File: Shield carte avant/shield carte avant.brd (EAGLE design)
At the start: 68.6 x 53.3 mm, 29 parts, among them IC1 MCP2562-E_P, IC2 MCP2515-I_P, J1 22-05-7078-07, J2 22-05-7028-02, J3 22-05-7038-03, J5 22-05-7028-02, M1 ARDUINO_R3_ICSP

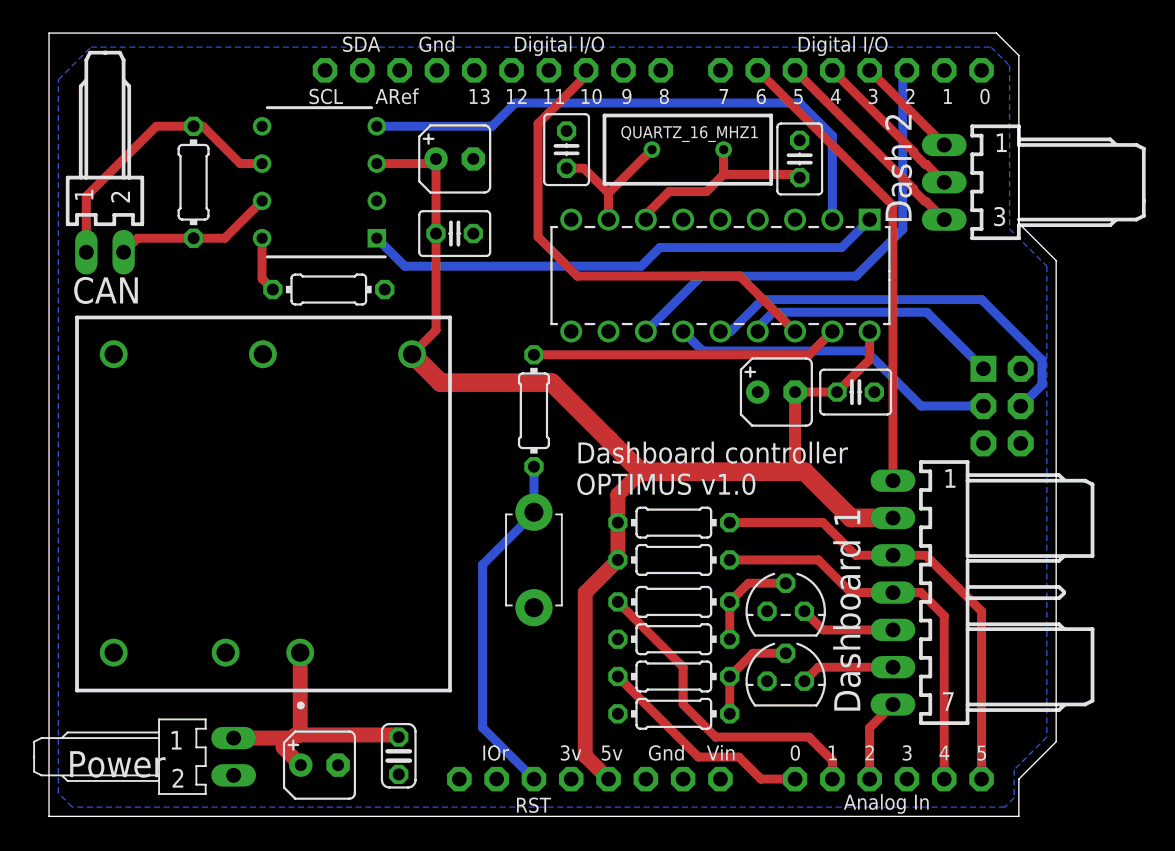
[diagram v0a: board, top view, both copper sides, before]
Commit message: Légères modifs avant envoie en prod
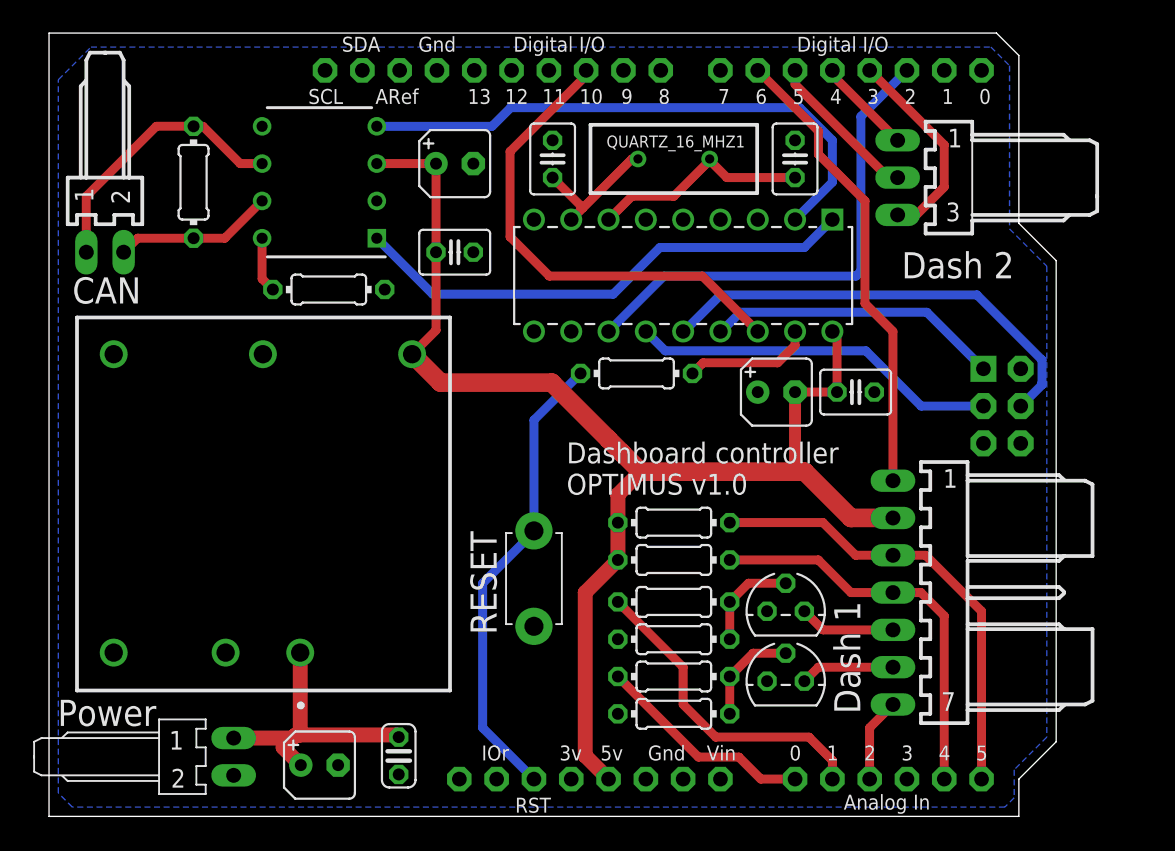
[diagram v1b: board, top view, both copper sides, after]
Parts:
- moved R4 7.43 mm to (41.3, 30.2), turned to 180 degrees
- moved J3 3.19 mm to (59.1, 43.5)
- moved IC2 2.54 mm to (34.3, 33.0)
- moved C10 1.27 mm to (28.9, 38.4)
- moved SW2 1.27 mm to (34.3, 16.2)
- moved C5 1.14 mm to (35.6, 44.8)
- moved QUARTZ_16_MHZ1 1.14 mm to (43.8, 44.8)
- moved C7 0.32 mm to (52.1, 44.8)
- moved C9 0.32 mm to (28.9, 44.5)
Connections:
- net SCL_SPI: now also J3.2; no longer J3.3
- net SDA_SPI: now also J3.1; no longer J3.2
- net TV: now also J3.3; no longer J3.1
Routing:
- net N$11: track 21.0 -> 8.73 mm
- net RESET: track 24.2 -> 31.8 mm
- net TV: track 7.18 -> 14.0 mm
- net SDA_SPI: track 10.8 -> 6.60 mm
- net SCL_SPI: track 14.4 -> 10.6 mm
- net SI: track 28.2 -> 31.1 mm
- net SCK: track 22.6 -> 25.1 mm
- net INT: track 31.3 -> 33.9 mm
- net SO: track 17.7 -> 20.0 mm
- net N$7: track 13.7 -> 15.0 mm
- net +5V: track 92.0 -> 90.8 mm
- net TXD: track 35.7 -> 34.7 mm
- net RXD: track 38.3 -> 38.9 mm
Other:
- board text added: "Dash 1"
- board text added: "RESET"
- board text removed: "Dashboard 1"
